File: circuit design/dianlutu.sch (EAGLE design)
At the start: 36 parts, among them U1 STM32-C-64, U2 LM386N-4/NOPB, X1 MINI-USB-SCHIELD-32005-201

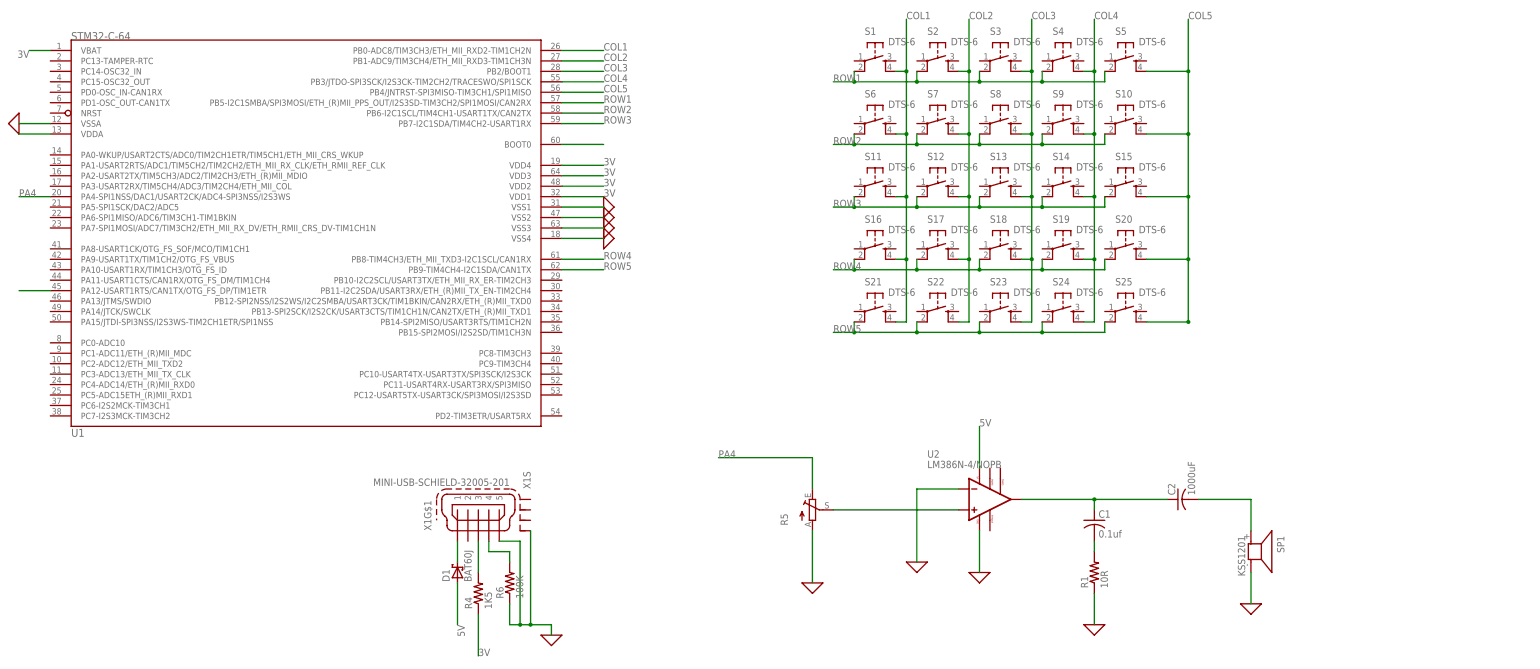
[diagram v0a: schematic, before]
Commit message: update files
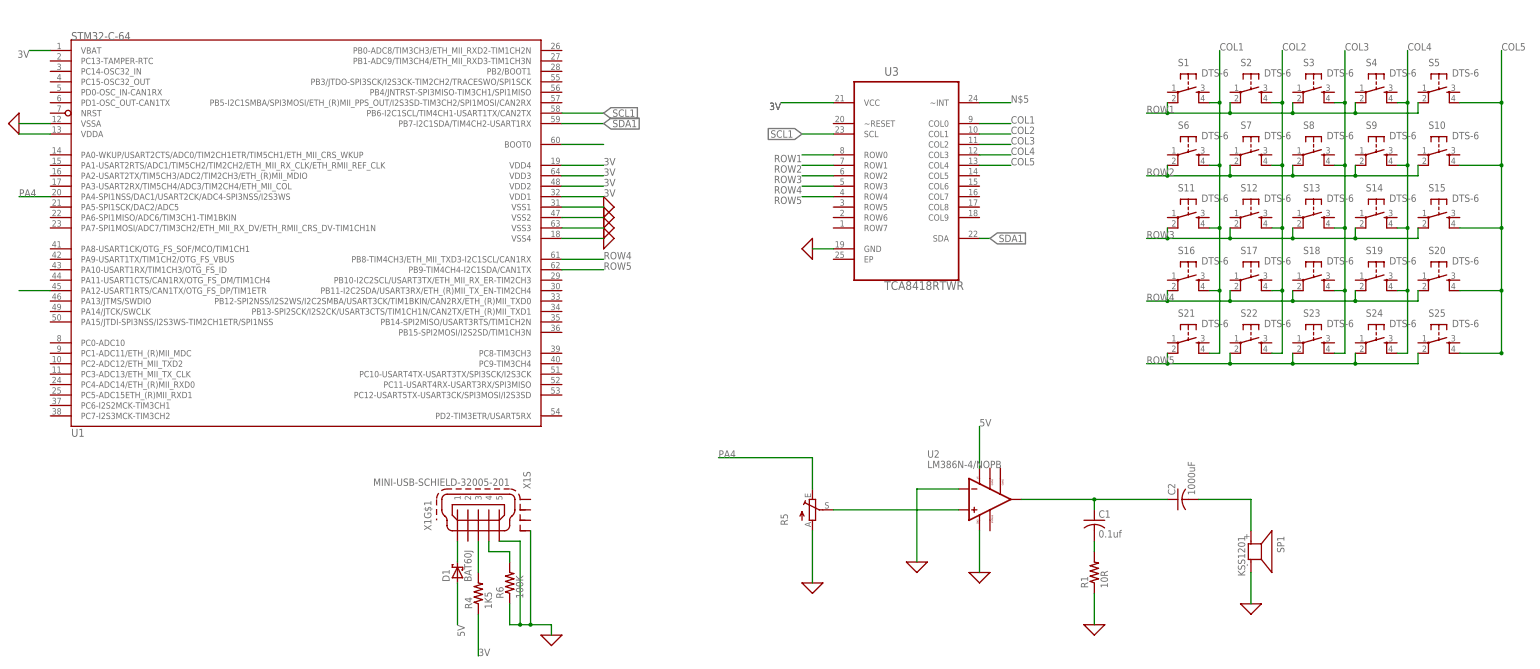
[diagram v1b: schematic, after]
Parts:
- added U3: TCA8418RTWR, TCA8418RTWR:TCA8418RTWR
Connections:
- new net N$5: U3.~INT
- new net SCL1: U1.PB6-I2C1SCL/TIM4CH1-USART1TX/CAN2TX, U3.SCL
- new net SDA1: U1.PB7-I2C1SDA/TIM4CH2-USART1RX, U3.SDA
- net 0: now also U3.GND
- net 3V: now also U3.VCC
- net COL1: now also U3.COL0; no longer U1.PB0-ADC8/TIM3CH3/ETH_MII_RXD2-TIM1CH2N
- net COL2: now also U3.COL1; no longer U1.PB1-ADC9/TIM3CH4/ETH_MII_RXD3-TIM1CH3N
- net COL3: now also U3.COL2; no longer U1.PB2/BOOT1
- net COL4: now also U3.COL3; no longer U1.PB3/JTDO-SPI3SCK/I2S3CK-TIM2CH2/TRACESWO/SPI1SCK
- net COL5: now also U3.COL4; no longer U1.PB4/JNTRST-SPI3MISO-TIM3CH1/SPI1MISO
- net ROW1: now also U3.ROW0; no longer U1.PB5-I2C1SMBA/SPI3MOSI/ETH_(R)MII_PPS_OUT/I2S3SD-TIM3CH2/SPI1MOSI/CAN2RX
- net ROW2: now also U3.ROW1; no longer U1.PB6-I2C1SCL/TIM4CH1-USART1TX/CAN2TX
- net ROW3: now also U3.ROW2; no longer U1.PB7-I2C1SDA/TIM4CH2-USART1RX
- net ROW4: now also U3.ROW3
- net ROW5: now also U3.ROW4
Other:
- moved on the sheet: S1, S10, S11, S12, S13, S14, S15, S16, S17, S18, S19, S2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
